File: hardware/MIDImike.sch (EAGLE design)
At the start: 5 parts, among them SW1 SPST, SW2 PUSH-BTN

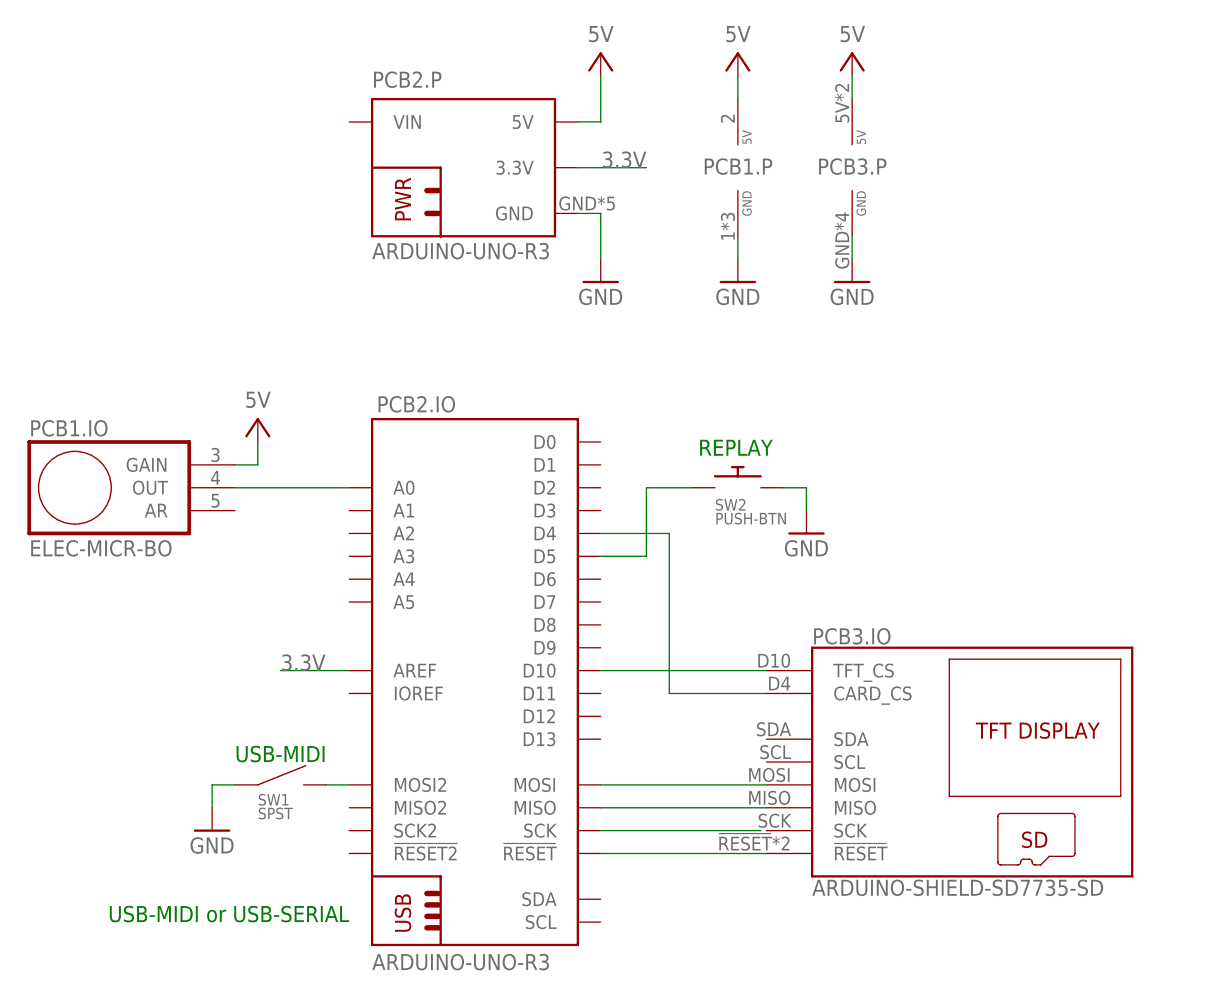
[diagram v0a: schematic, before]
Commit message: spring clean
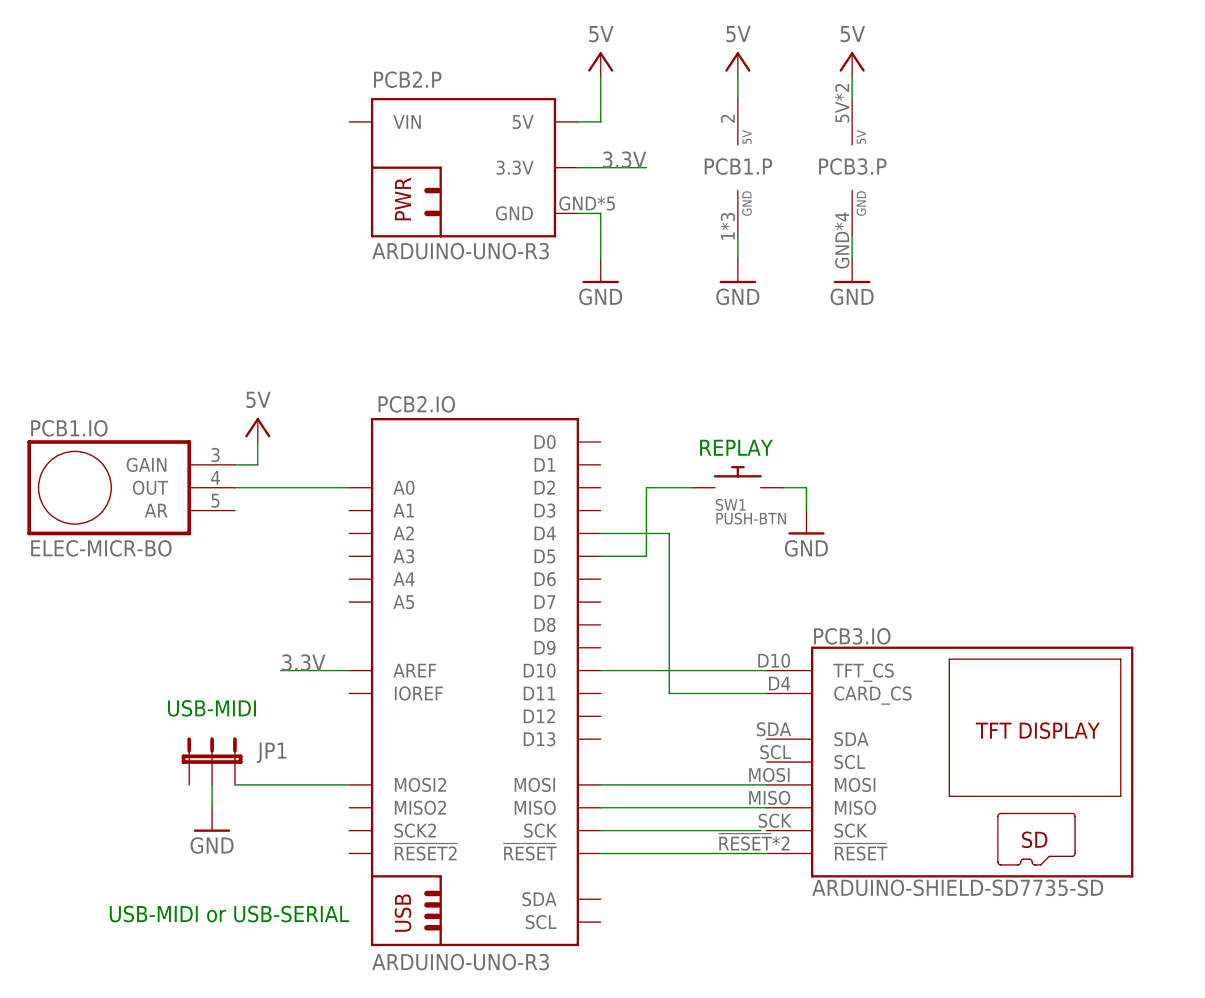
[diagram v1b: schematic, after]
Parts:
- removed SW2: PUSH-BTN, Coert-Vonk:PUSH-BTN
- added JP1: (no value), Coert-Vonk:JP2E
- SW1: value SPST -> PUSH-BTN; device Coert-Vonk:SPST -> Coert-Vonk:PUSH-BTN
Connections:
- net N$1 renamed A0
- removed net N$10: PCB1.IO.GAIN
- removed net N$8: PCB2.IO.D5, SW2.1
- new net REPLAY: PCB2.IO.D5, SW1.1
- net 5V: now also PCB1.IO.GAIN
- net GND: now also JP1.2; no longer SW2.2
- net N$3: now also JP1.3; no longer SW1.1
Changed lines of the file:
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@@
 <part name="GND2" library="Coert-Vonk" deviceset="GND" device=""/>
 <part name="GND3" library="Coert-Vonk" deviceset="GND" device=""/>
-<part name="SW2" library="Coert-Vonk" deviceset="PUSH-BTN" device=""/>
-<part name="SW1" library="Coert-Vonk" deviceset="SPST" device=""/>
+<part name="SW1" library="Coert-Vonk" deviceset="PUSH-BTN" device=""/>
 <part name="GND5" library="Coert-Vonk" deviceset="GND" device=""/>
 <part name="GND6" library="Coert-Vonk" deviceset="GND" device=""/>
@@
 <part name="PCB2" library="Coert-Vonk" deviceset="ARDUINO-UNO-R3" device=""/>
 <part name="P+4" library="Coert-Vonk" deviceset="5V" device=""/>
+<part name="JP1" library="Coert-Vonk" deviceset="JP2E" device="" package3d_urn="urn:adsk.eagle:package:15452/1"/>
 </parts>
 <sheets>
 <sheet>
 <plain>
-<text x="43.18" y="83.82" size="1.778" layer="91">USB-MIDI</text>
+<text x="40.64" y="88.9" size="1.778" layer="91" align="bottom-center">USB-MIDI</text>
 <text x="98.806" y="117.856" size="1.778" layer="91" align="bottom-center">REPLAY</text>
 <text x="55.88" y="66.04" size="1.778" layer="91" align="bottom-right">USB-MIDI or USB-SERIAL</text>
@@
 <attribute name="VALUE" x="99.06" y="134.62" size="1.778" layer="96" align="bottom-center"/>
 </instance>
-<instance part="SW2" gate="G$1" x="99.06" y="114.3" smashed="yes">
+<instance part="SW1" gate="G$1" x="99.06" y="114.3" smashed="yes">
 <attribute name="NAME" x="96.518090625" y="111.76381875" size="1.27" layer="95"/>
 <attribute name="VALUE" x="96.518190625" y="110.232390625" size="1.27" layer="96"/>
-</instance>
-<instance part="SW1" gate="G$1" x="48.26" y="81.28" smashed="yes">
-<attribute name="NAME" x="45.72" y="78.994" size="1.27" layer="95"/>
-<attribute name="VALUE" x="45.72" y="78.74" size="1.27" layer="96" align="top-left"/>
 </instance>
 <instance part="GND5" gate="1" x="40.64" y="76.2" smashed="yes">
@@
 <instance part="P+4" gate="1" x="45.72" y="121.92" smashed="yes">
 <attribute name="VALUE" x="45.72" y="123.19" size="1.778" layer="96" align="bottom-center"/>
+</instance>
+<instance part="JP1" gate="1" x="40.64" y="83.82" smashed="yes">
+<attribute name="NAME" x="45.72" y="85.09" size="1.778" layer="95" rot="R180" align="center-right"/>
+<attribute name="VALUE" x="46.355" y="83.82" size="1.778" layer="96" rot="R90"/>
 </instance>
 </instances>
@@
 </segment>
 <segment>
-<pinref part="GND5" gate="1" pin="GND"/>
-<wire x1="40.64" y1="78.74" x2="40.64" y2="81.28" width="0.1524" layer="91"/>
 <pinref part="SW1" gate="G$1" pin="2"/>
-<wire x1="40.64" y1="81.28" x2="43.18" y2="81.28" width="0.1524" layer="91"/>
-</segment>
-<segment>
-<pinref part="SW2" gate="G$1" pin="2"/>
 <wire x1="104.14" y1="114.3" x2="106.68" y2="114.3" width="0.1524" layer="91"/>
 <wire x1="106.68" y1="114.3" x2="106.68" y2="111.76" width="0.1524" layer="91"/>
 <pinref part="GND6" gate="1" pin="GND"/>
+</segment>
+<segment>
+<pinref part="GND5" gate="1" pin="GND"/>
+<pinref part="JP1" gate="1" pin="2"/>
+<wire x1="40.64" y1="81.28" x2="40.64" y2="78.74" width="0.1524" layer="91"/>
 </segment>
 </net>
@@
 <wire x1="111.76" y1="160.02" x2="111.76" y2="157.48" width="0.1524" layer="91"/>
 </segment>
-</net>
-<net name="N$1" class="0">
+<segment>
+<pinref part="PCB1" gate=".IO" pin="GAIN"/>
+<pinref part="P+4" gate="1" pin="5V"/>
+<wire x1="43.18" y1="116.84" x2="45.72" y2="116.84" width="0.1524" layer="91"/>
+<wire x1="45.72" y1="116.84" x2="45.72" y2="119.38" width="0.1524" layer="91"/>
+</segment>
+</net>
+<net name="A0" class="0">
 <segment>
 <wire x1="43.18" y1="114.3" x2="55.88" y2="114.3" width="0.1524" layer="91"/>
@@
 </segment>
 </net>
-<net name="N$3" class="0">
-<segment>
-<pinref part="SW1" gate="G$1" pin="1"/>
-<wire x1="53.34" y1="81.28" x2="55.88" y2="81.28" width="0.1524" layer="91"/>
-<pinref part="PCB2" gate=".IO" pin="MOSI2"/>
-</segment>
-</net>
-<net name="N$8" class="0">
+<net name="REPLAY" class="0">
 <segment>
 <wire x1="83.82" y1="106.68" x2="88.9" y2="106.68" width="0.1524" layer="91"/>
 <wire x1="88.9" y1="106.68" x2="88.9" y2="114.3" width="0.1524" layer="91"/>
-<pinref part="SW2" gate="G$1" pin="1"/>
+<pinref part="SW1" gate="G$1" pin="1"/>
 <wire x1="88.9" y1="114.3" x2="93.98" y2="114.3" width="0.1524" layer="91"/>
 <pinref part="PCB2" gate=".IO" pin="D5"/>
 </segment>
 </net>
-<net name="N$10" class="0">
-<segment>
-<wire x1="43.18" y1="116.84" x2="45.72" y2="116.84" width="0.1524" layer="91"/>
-<pinref part="PCB1" gate=".IO" pin="GAIN"/>
-<pinref part="P+4" gate="1" pin="5V"/>
-<wire x1="45.72" y1="119.38" x2="45.72" y2="116.84" width="0.1524" layer="91"/>
+<net name="N$3" class="0">
+<segment>
+<pinref part="PCB2" gate=".IO" pin="MOSI2"/>
+<pinref part="JP1" gate="1" pin="3"/>
+<wire x1="55.88" y1="81.28" x2="43.18" y2="81.28" width="0.1524" layer="91"/>
 </segment>
 </net>
@@
 </drawing>
 <compatibility>
+<note version="8.3" severity="warning">
+Since Version 8.3, EAGLE supports URNs for individual library
+assets (packages, symbols, and devices). The URNs of those assets
+will not be understood (or retained) with this version.
+</note>
+<note version="8.3" severity="warning">
+Since Version 8.3, EAGLE supports the association of 3D packages
+with devices in libraries, schematics, and board files. Those 3D
+packages will not be understood (or retained) with this version.
+</note>
 <note version="9.0" severity="warning">
 Since Version 9.0, EAGLE supports the align property for labels.
